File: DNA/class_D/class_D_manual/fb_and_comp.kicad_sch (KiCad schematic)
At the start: 1 part, among them U4 OPA859

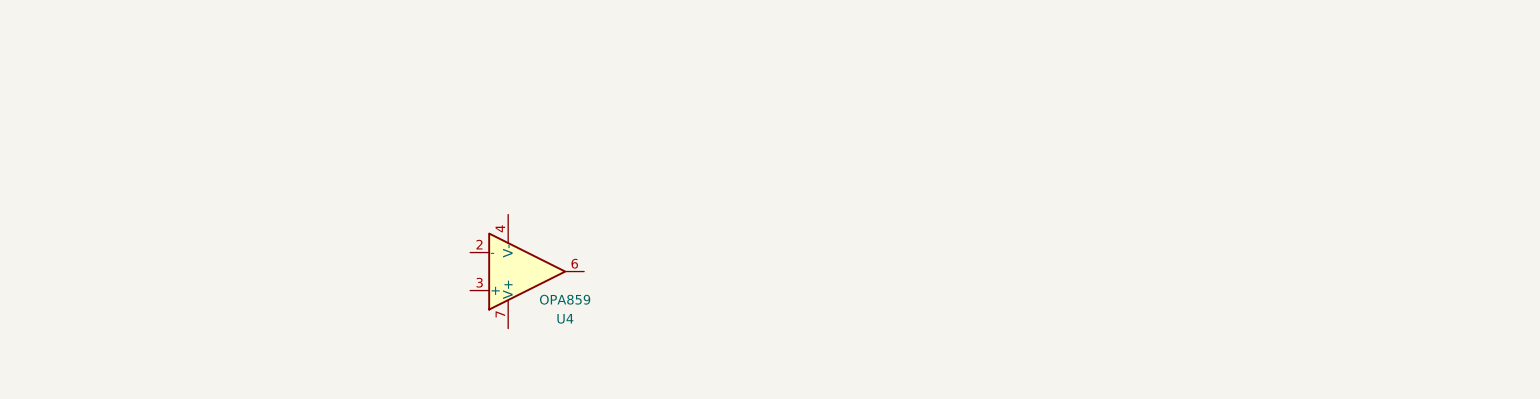
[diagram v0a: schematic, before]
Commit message: [DNA]: class D, more of schematics added.
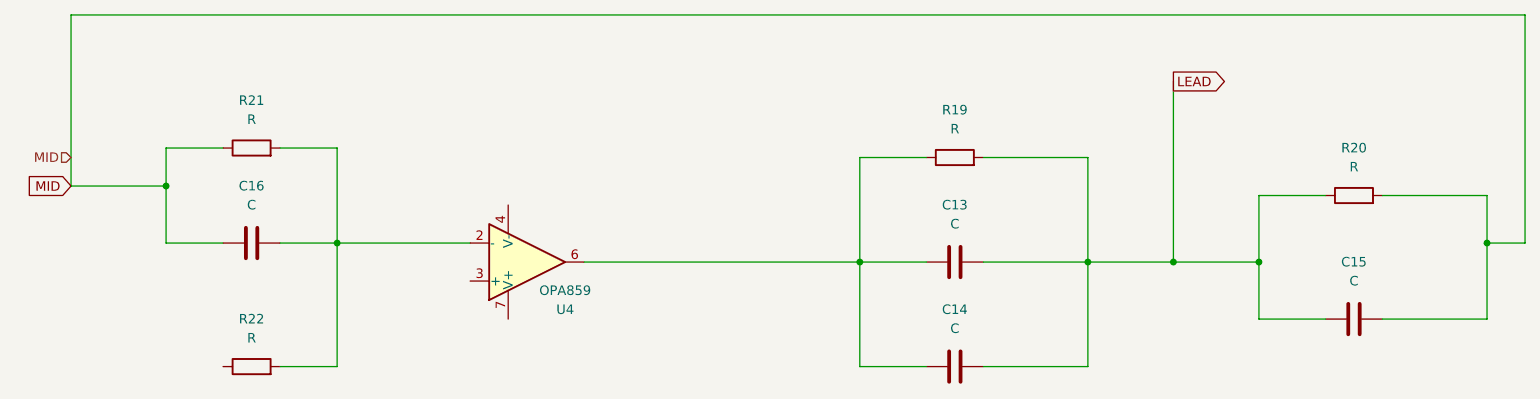
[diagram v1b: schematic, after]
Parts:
- added C13, C14, C15, C16: C, symbol Device:C
- added R19, R20, R21, R22: R, symbol Device:R
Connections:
- net at U4.2 (-): now also C16.2, R21.2, R22.2
- net at U4.6: now also C13.1, C14.1, R19.1
- new net LEAD: C13.2, C14.2, C15.1, R19.2, R20.1
- new net MID: C15.2, C16.1, R20.2, R21.1
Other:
- moved on the sheet: U4
